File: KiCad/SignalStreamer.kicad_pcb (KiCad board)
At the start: 2 copper layers, 100.3 x 59.1 mm, 46 parts, among them J105 Conn_01x02, T101 Coupled_Inductors_2

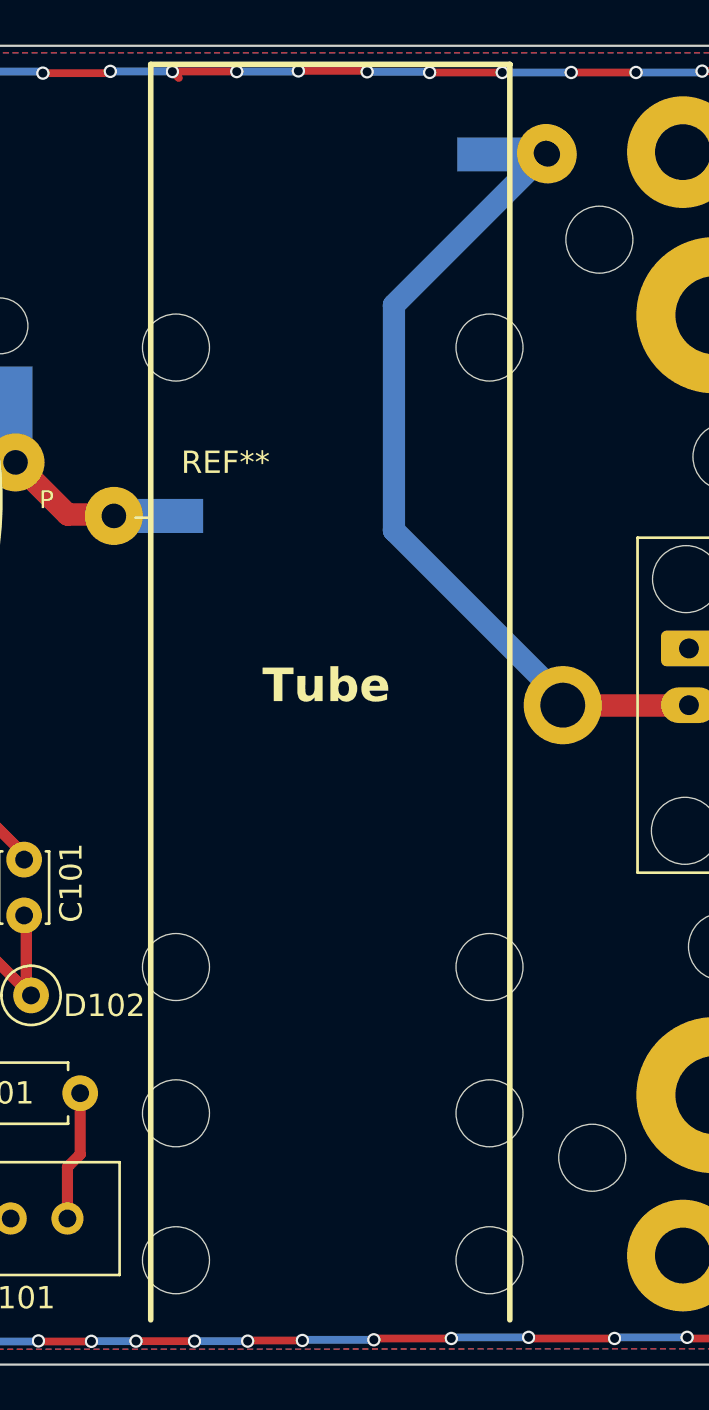
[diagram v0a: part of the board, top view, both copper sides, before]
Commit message: Development
PCB Updates
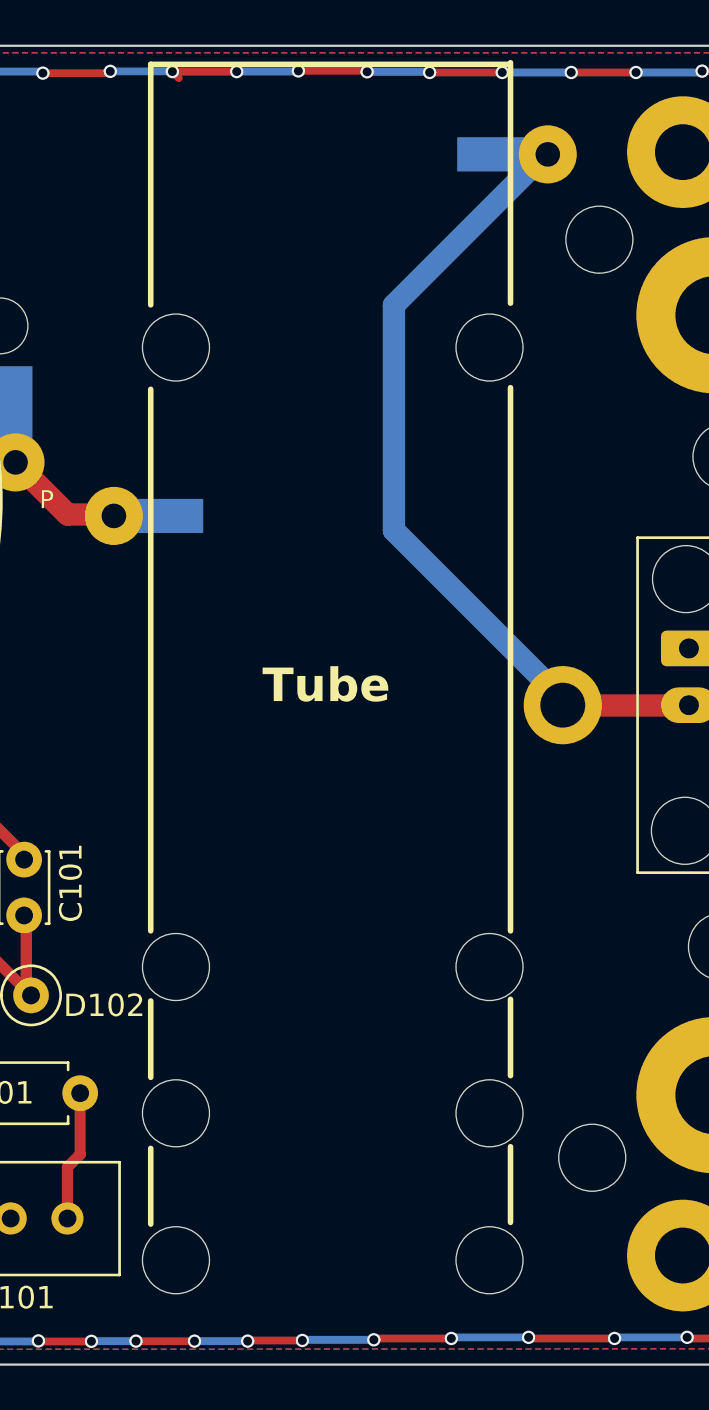
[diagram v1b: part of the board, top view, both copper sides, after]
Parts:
- removed the L101 at (120.6, 63.3)
- L101: renamed from REF**; value L_Lipstick_Tube_Variable -> FB-31-4852
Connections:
- L101 pad 1: (no net) -> Net-(T101-OUT1B)
- L101 pad 2: (no net) -> Net-(J105-Pin_1)
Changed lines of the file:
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@@
 			)
 		)
+		(property "Digi-Key Part No." ""
+			(at 0 0 0)
+			(unlocked yes)
+			(layer "F.Fab")
+			(hide yes)
+			(effects
+				(font
+					(size 1 1)
+					(thickness 0.15)
+				)
+			)
+		)
 		(sheetname "/")
 		(sheetfile "SignalStreamer.kicad_sch")
@@
 			(pinfunction "OUT1A")
 			(pintype "passive")
+			(clearance 0.5)
 			(zone_connect 2)
 		)
@@
 			(pinfunction "OUT1B")
 			(pintype "passive")
+			(clearance 0.5)
 			(zone_connect 2)
 		)
@@
 			)
 		)
-		(property "Datasheet" ""
+		(property "Datasheet" "~"
 			(at 0 0 90)
 			(layer "F.Fab")
@@
 			)
 		)
-		(property "Description" "CONN BNC JACK R/A 50 OHM PCB"
+		(property "Description" "Generic connector, single row, 01x02, script generated (kicad-library-utils/schlib/autogen/connector/)"
 			(at 37.8625 216.6875 0)
 			(layer "F.Fab")
@@
 			)
 		)
-		(property "Link" "https://www.digikey.com/en/products/detail/amphenol-rf/31-5431/80179?utm_adgroup=Coaxial%20Connectors%20%28RF%29&utm_source=google&utm_medium=cpc&utm_campaign=Shopping_Product_Connectors%2C%20Interconnects&utm_term=&utm_content=Coaxial%20Connectors%20%28RF%29&gclid=Cj0KCQjw1rqkBhCTARIsAAHz7K07BKQI4hz-lx2UKWOAkhojF887qRyZwSAGP9HUwnWBejkHZJLi92kaAsMsEALw_wcB"
+		(property "Link" ""
 			(at 37.8625 216.6875 0)
 			(layer "F.Fab")
@@
 			)
 		)
-		(property "Manufacturer" "Amphenol RF"
+		(property "Manufacturer" ""
 			(at 37.8625 216.6875 0)
 			(layer "F.Fab")
@@
 			)
 		)
-		(property "Manufacturer PN" "31-5431"
+		(property "Manufacturer PN" ""
 			(at 37.8625 216.6875 0)
 			(layer "F.Fab")
@@
 			)
 		)
+		(property "Sim.Device" ""
+			(at 0 0 270)
+			(unlocked yes)
+			(layer "F.Fab")
+			(hide yes)
+			(effects
+				(font
+					(size 1 1)
+					(thickness 0.15)
+				)
+			)
+		)
+		(property "Sim.Pins" ""
+			(at 0 0 270)
+			(unlocked yes)
+			(layer "F.Fab")
+			(hide yes)
+			(effects
+				(font
+					(size 1 1)
+					(thickness 0.15)
+				)
+			)
+		)
 		(property ki_fp_filters "Connector*:*_1x??_*")
 		(sheetname "/")
 		(sheetfile "SignalStreamer.kicad_sch")
-		(attr through_hole)
+		(attr through_hole exclude_from_bom)
 		(fp_line
 			(start -7.5 2.3)
@@
 	(footprint ""
 		(layer "F.Cu")
-		(at 120.58 63.31 -90)
-		(property "Reference" "L101"
-			(at 0 0 90)
-			(layer "F.SilkS")
-			(hide yes)
-			(effects
-				(font
-					(size 1.27 1.27)
-					(thickness 0.15)
-				)
-			)
-		)
-		(property "Value" "0.4-1.0uH"
-			(at 0 0 90)
-			(layer "F.Fab")
-			(effects
-				(font
-					(size 1.27 1.27)
-					(thickness 0.15)
-				)
-			)
-		)
-		(property "Datasheet" ""
-			(at 0 0 90)
-			(layer "F.Fab")
-			(hide yes)
-			(effects
-				(font
-					(size 1.27 1.27)
-					(thickness 0.15)
-				)
-			)
-		)
-		(property "Description" ""
-			(at 0 0 90)
-			(layer "F.Fab")
-			(hide yes)
-			(effects
-				(font
-					(size 1.27 1.27)
-					(thickness 0.15)
-				)
-			)
-		)
-		(sheetname "/")
-		(sheetfile "SignalStreamer.kicad_sch")
-		(pad "2" thru_hole circle
-			(at 0 0 270)
-			(size 2.6 2.6)
-			(drill 1.1)
-			(layers "*.Cu" "*.Mask")
-			(remove_unused_layers no)
-			(net 15 "Net-(J105-Pin_1)")
-			(pinfunction "2")
-			(pintype "passive")
-			(clearance 0.5)
-			(zone_connect 2)
-		)
-		(embedded_fonts no)
-	)
-	(footprint ""
-		(layer "F.Cu")
 		(at 122.97 67.19)
 		(property "Reference" ""
@@
 		(descr "Inductor, Axial series, Axial, Horizontal, pin pitch=10.16mm, length*diameter=6.6*2.7mm^2, Vishay, IM-2, http://www.vishay.com/docs/34030/im.pdf")
 		(tags "Inductor Axial series Axial Horizontal pin pitch 10.16mm  length 6.6mm diameter 2.7mm Vishay IM-2")
-		(property "Reference" "REF**"
+		(property "Reference" "L101"
 			(at 5.08 -2.47 0)
 			(layer "F.SilkS")
+			(hide yes)
 			(effects
 				(font
@@
 			)
 		)
-		(property "Value" "L_Lipstick_Tube_Variable"
+		(property "Value" "FB-31-4852"
 			(at 5.08 2.47 0)
 			(layer "F.Fab")
+			(hide yes)
 			(effects
 				(font
@@
 			)
 		)
-		(property "Description" ""
+		(property "Description" "Lipstick tube variable inductor"
 			(at 0 0 0)
 			(layer "F.Fab")
@@
 			)
 		)
+		(property "Digi-Key Part No." ""
+			(at 0 0 0)
+			(unlocked yes)
+			(layer "F.Fab")
+			(hide yes)
+			(effects
+				(font
+					(size 1 1)
+					(thickness 0.15)
+				)
+			)
+		)
+		(property "Link" ""
+			(at 0 0 0)
+			(unlocked yes)
+			(layer "F.Fab")
+			(hide yes)
+			(effects
+				(font
+					(size 1 1)
+					(thickness 0.15)
+				)
+			)
+		)
+		(property "Manufacturer" "Amidon"
+			(at 0 0 0)
+			(unlocked yes)
+			(layer "F.Fab")
+			(hide yes)
+			(effects
+				(font
+					(size 1 1)
+					(thickness 0.15)
+				)
+			)
+		)
+		(property "Manufacturer PN" "FB-31-4852"
+			(at 0 0 0)
+			(unlocked yes)
+			(layer "F.Fab")
+			(hide yes)
+			(effects
+				(font
+					(size 1 1)
+					(thickness 0.15)
+				)
+			)
+		)
+		(sheetname "/")
+		(sheetfile "SignalStreamer.kicad_sch")
 		(attr through_hole)
 		(fp_line
-			(start 1.04 0)
-			(end 1.66 0)
+			(start 1.73 -20.3)
+			(end 1.73 -9.53)
 			(stroke
-				(width 0.12)
+				(width 0.25)
 				(type solid)
 			)
@@
 		)
 		(fp_line
-			(start 1.73 35.92)
-			(end 1.73 -20.3)
+			(start 1.73 -5.75)
+			(end 1.73 18.5)
+			(stroke
+				(width 0.25)
+				(type solid)
+			)
+			(layer "F.SilkS")
+		)
+		(fp_line
+			(start 1.73 21.64)
+			(end 1.73 25.06)
+			(stroke
+				(width 0.25)
+				(type solid)
+			)
+			(layer "F.SilkS")
+		)
+		(fp_line
+			(start 1.73 28.24)
+			(end 1.73 31.63)
 			(stroke
 				(width 0.25)
@@
 		)
 		(fp_line
-			(start 17.81 -20.3)
-			(end 17.81 35.92)
+			(start 17.84 -20.375)
+			(end 17.84 -9.605)
+			(stroke
+				(width 0.25)
+				(type solid)
+			)
+			(layer "F.SilkS")
+		)
+		(fp_line
+			(start 17.84 -5.825)
+			(end 17.84 18.5)
+			(stroke
+				(width 0.25)
+				(type solid)
+			)
+			(layer "F.SilkS")
+		)
+		(fp_line
+			(start 17.84 21.565)
+			(end 17.84 24.985)
+			(stroke
+				(width 0.25)
+				(type solid)
+			)
+			(layer "F.SilkS")
+		)
+		(fp_line
+			(start 17.84 28.165)
+			(end 17.84 31.555)
 			(stroke
 				(width 0.25)
@@
 			(layers "*.Cu" "*.Mask")
 			(remove_unused_layers no)
+			(net 9 "Net-(T101-OUT1B)")
+			(pinfunction "1")
+			(pintype "passive")
 			(clearance 0.5)
 			(zone_connect 2)
@@
 			(size 1.524 5)
 			(layers "B.Cu" "B.Mask" "B.Paste")
+			(net 9 "Net-(T101-OUT1B)")
+			(pinfunction "1")
+			(pintype "passive")
 			(zone_connect 2)
 		)
@@
 			(size 1.524 5)
 			(layers "B.Cu" "B.Mask" "B.Paste")
+			(net 15 "Net-(J105-Pin_1)")
+			(pinfunction "2")
+			(pintype "passive")
 			(clearance 0.5)
 			(zone_connect 2)
@@
 			(layers "*.Cu" "*.Mask")
 			(remove_unused_layers no)
+			(net 15 "Net-(J105-Pin_1)")
+			(pinfunction "2")
+			(pintype "passive")
 			(clearance 0.5)
 			(zone_connect 2)
@@
 			)
 		)
-		(property "Datasheet" ""
+		(property "Datasheet" "https://www.st.com/content/ccc/resource/technical/document/datasheet/a8/9d/10/57/ac/a3/4f/81/CD00000759.pdf/files/CD00000759.pdf/jcr:content/translations/en.CD00000759.pdf"
 			(at 0 0 0)
 			(layer "F.Fab")
@@
 			)
 		)
-		(property "Description" ""
+		(property "Description" "RF DIODE SCHOTTKY 70V 430MW DO35"
 			(at 0 0 0)
 			(layer "F.Fab")
@@
 			)
 		)
-		(property "Datasheet" ""
+		(property "Datasheet" "https://www.st.com/content/ccc/resource/technical/document/datasheet/a8/9d/10/57/ac/a3/4f/81/CD00000759.pdf/files/CD00000759.pdf/jcr:content/translations/en.CD00000759.pdf"
 			(at 0 0 180)
 			(layer "F.Fab")
@@
 			)
 		)
-		(property "Description" ""
+		(property "Description" "RF DIODE SCHOTTKY 70V 430MW DO35"
 			(at 0 0 180)
 			(layer "F.Fab")
@@
 	)
 	(zone
-		(net 0)
-		(net_name "")
-		(layer "F.Cu")
-		(hatch edge 0.5)
-		(connect_pads
-			(clearance 0)
-		)
-		(min_thickness 0.25)
-		(filled_areas_thickness no)
-		(keepout
-			(tracks not_allowed)
-			(vias not_allowed)
-			(pads not_allowed)
-			(copperpour allowed)
-			(footprints allowed)
-		)
-		(placement
-			(enabled no)
-			(sheetname "")
-		)
-		(fill
-			(thermal_gap 0.5)
-			(thermal_bridge_width 0.5)
-		)
-		(polygon
-			(pts
-				(xy 103.15 63.5) (xy 118.54 63.52) (xy 118.54 80.29) (xy 102.76 80.1) (xy 102.95 63.33)
-			)
-		)
-	)
-	(zone
 		(net 4)
 		(net_name "GND")
@@
 			(tracks not_allowed)
 			(vias not_allowed)
-			(pads not_allowed)
+			(pads allowed)
 			(copperpour not_allowed)
 			(footprints allowed)
